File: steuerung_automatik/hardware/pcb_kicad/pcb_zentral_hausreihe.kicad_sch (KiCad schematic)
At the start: 3 parts, among them J201 weidmueller_SL5.08HC-12-90, U201 shiftregister_74HC595

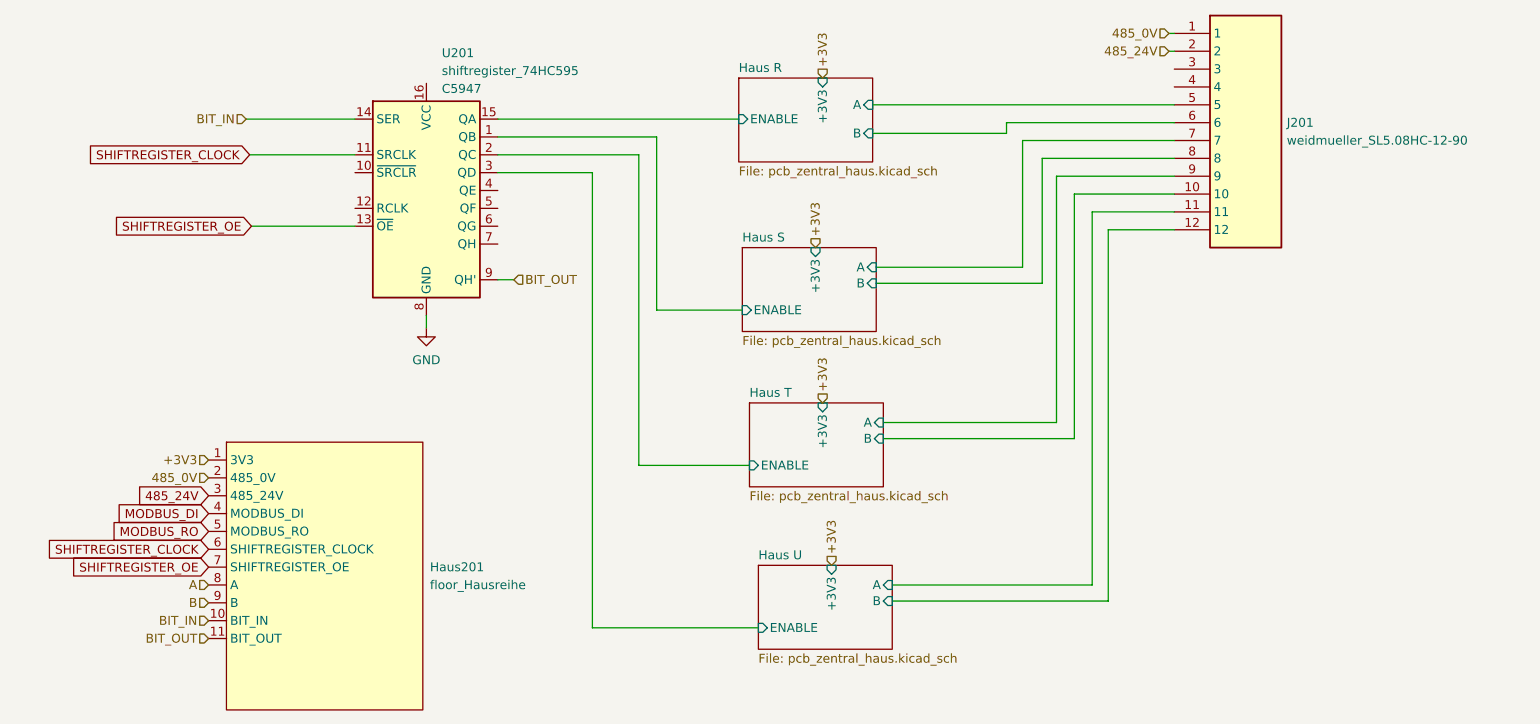
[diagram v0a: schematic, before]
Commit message: Nach Review
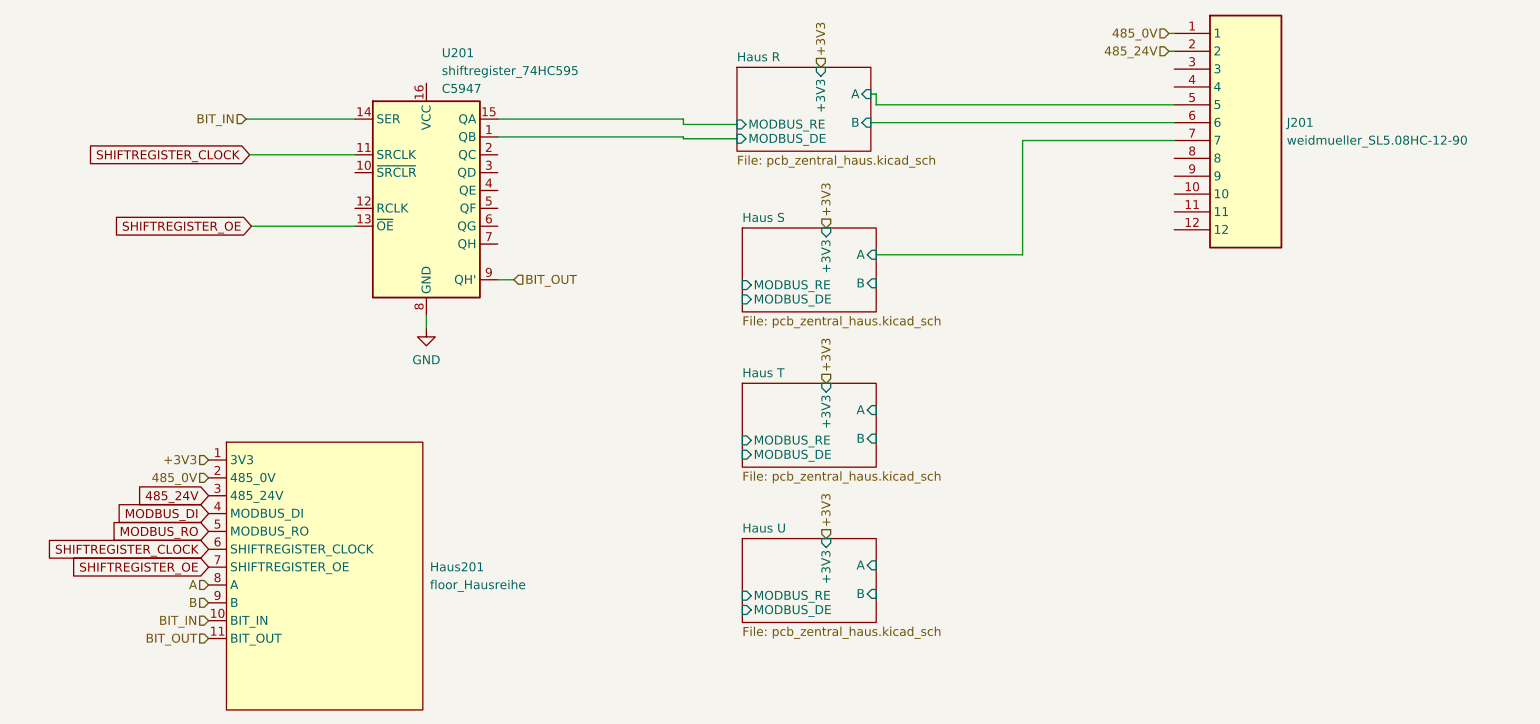
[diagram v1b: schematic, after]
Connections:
- net Haus S/B: no longer J201.8
- net Haus T/A: no longer J201.9
- net Haus T/B: no longer J201.10
- net Haus U/A: no longer J201.11
- net Haus U/B: no longer J201.12
- net Haus R/ENABLE renamed Haus R/MODBUS_RE
- net Haus S/ENABLE renamed Haus R/MODBUS_DE
- net Haus T/ENABLE: no longer names the net of U201.2 (QC)
- net Haus U/ENABLE: no longer names the net of U201.3 (QD)
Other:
- sheet Haus R ports: added MODBUS_DE, MODBUS_RE; removed ENABLE
- sheet Haus S ports: added MODBUS_DE, MODBUS_RE; removed ENABLE
- sheet Haus T ports: added MODBUS_DE, MODBUS_RE; removed ENABLE
- sheet Haus U ports: added MODBUS_DE, MODBUS_RE; removed ENABLE
